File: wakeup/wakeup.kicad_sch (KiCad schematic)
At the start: 15 parts, among them J1 Connector, U1 74HC00, U2 74HC393

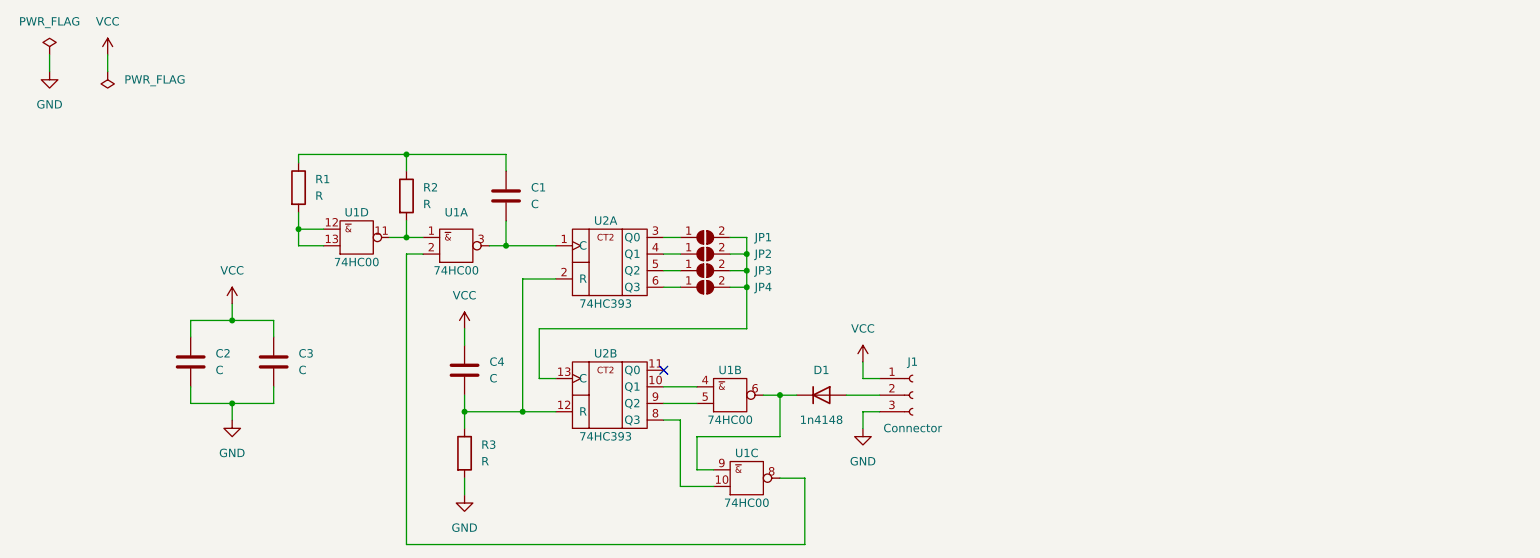
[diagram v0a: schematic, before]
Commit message: non functional update
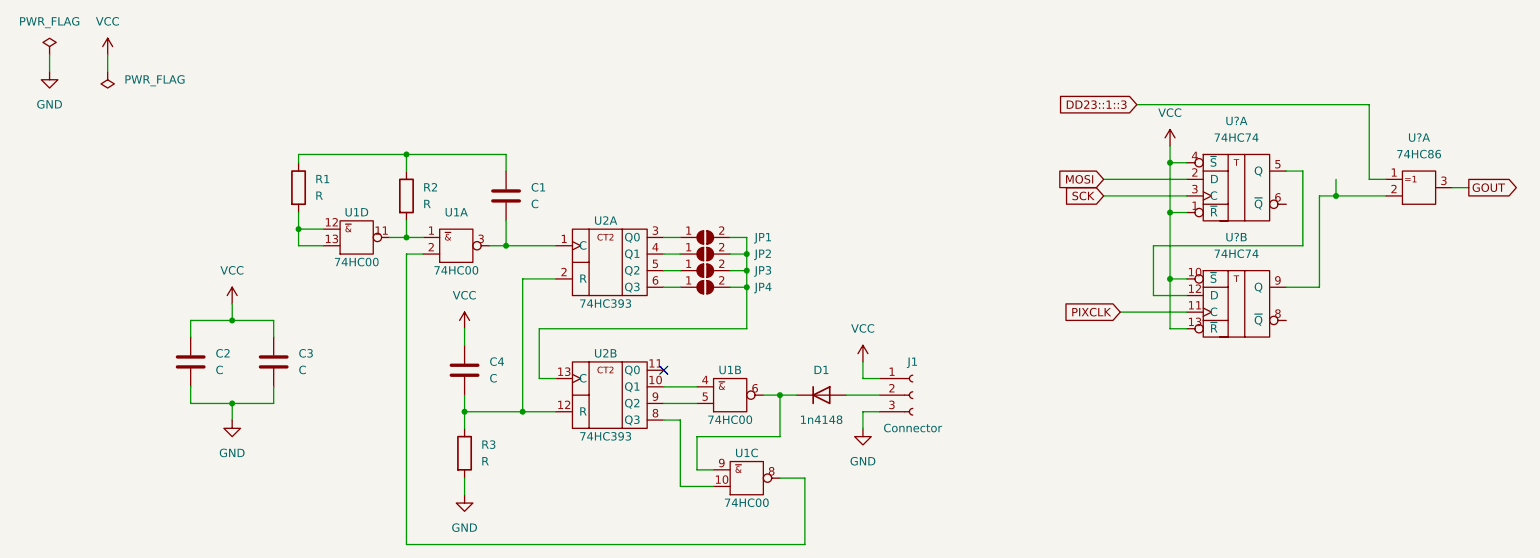
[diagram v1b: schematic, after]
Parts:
- added U? (x2): 74HC74, symbol 74IEC:74HC74
- added U?: 74HC86, symbol 74IEC:74HC86
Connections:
- net GND: now also U?.7 (GND), U?.7 (GND), U?.7 (GND)
- net VCC: now also U?.1 (~{R}), U?.10 (~{S}), U?.13 (~{R}), U?.14 (VCC), U?.14 (VCC), U?.14 (VCC), U?.4 (~{S})
- new net: U?.12 (D), U?.5 (Q)
- new net: U?.2 (B), U?.9 (Q)
- new net DD23::1::3: U?.1 (A)
- new net GOUT: U?.3 (Y)
- new net MOSI: U?.2 (D)
- new net PIXCLK: U?.11 (C)
- new net SCK: U?.3 (C)
